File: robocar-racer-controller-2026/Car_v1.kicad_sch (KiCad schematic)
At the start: 36 parts, among them J1 GY-87, J10 Buck in, J11 Motor_in, J12 Bateria 3s, J13 Buck_out, J14 Raspbery_usbc, J15 Step_up, J16 Radio, J3 Sinal_Servo, J4 Sinal_Motor, J5 Conn_01x19_Socket, J6 Conn_01x19_Socket, J7 Serial, J8 ADS1115, J9 Bateria 2s, SW1 SW_DPST_x2, SW2 SW_DPST_x2, U2 ESP32-DEVKITC-32D

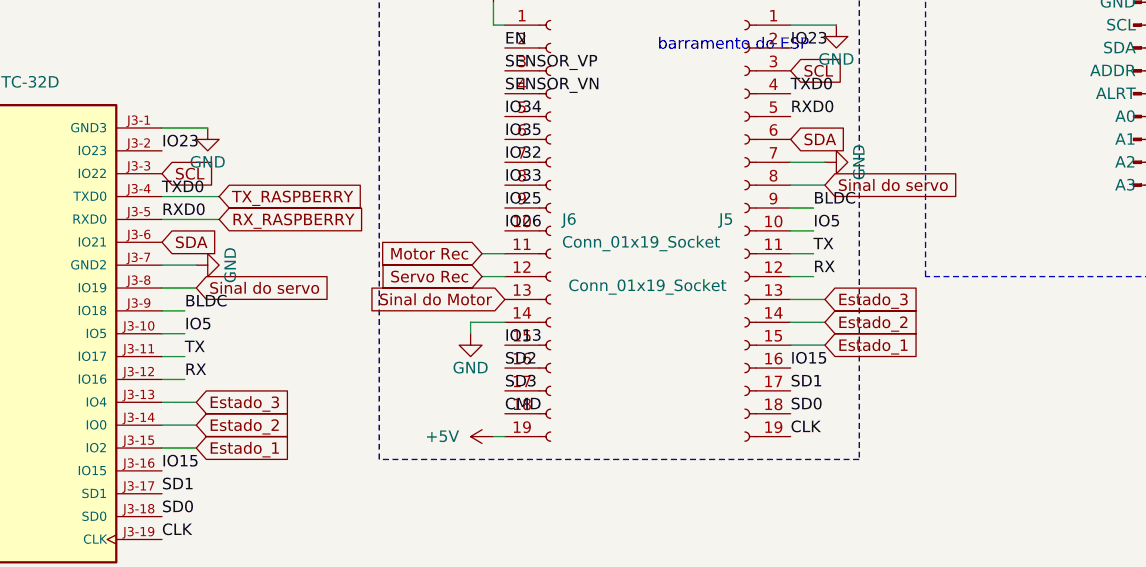
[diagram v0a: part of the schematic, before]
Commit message: ajustes na entrada serial
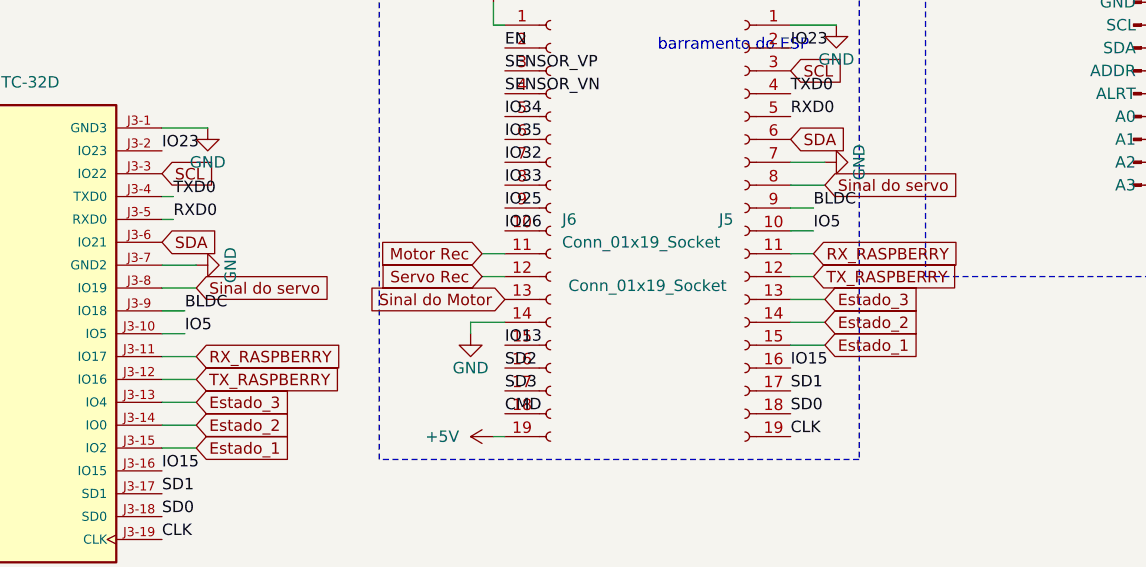
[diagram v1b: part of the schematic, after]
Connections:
- net RX is gone; now on net TX_RASPBERRY: J5.12 (Pin_12), U2.J3-12 (IO16)
- net TX is gone; now on net RX_RASPBERRY: J5.11 (Pin_11), U2.J3-11 (IO17)
- net RX_RASPBERRY: no longer J5.5 (Pin_5), U2.J3-5 (RXD0)
- net TX_RASPBERRY: no longer J5.4 (Pin_4), U2.J3-4 (TXD0)
- new net RXD0: J5.5 (Pin_5), U2.J3-5 (RXD0)
- new net TXD0: J5.4 (Pin_4), U2.J3-4 (TXD0)
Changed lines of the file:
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@@
-	(wire
-		(pts
-			(xy 132.08 135.89) (xy 138.43 135.89)
-		)
-		(stroke
-			(width 0)
-			(type default)
-		)
-	)
 	(wire
 		(pts
@@
 	(wire
 		(pts
+			(xy 132.08 156.21) (xy 135.89 156.21)
+		)
+		(stroke
+			(width 0)
+			(type default)
+		)
+	)
+	(wire
+		(pts
+			(xy 132.08 153.67) (xy 135.89 153.67)
+		)
+		(stroke
+			(width 0)
+			(type default)
+		)
+	)
+	(wire
+		(pts
 			(xy 168.91 116.84) (xy 170.18 116.84)
 		)
@@
 	(wire
 		(pts
+			(xy 133.35 138.43) (xy 132.08 138.43)
+		)
+		(stroke
+			(width 0)
+			(type default)
+		)
+	)
+	(wire
+		(pts
 			(xy 62.23 124.46) (xy 62.23 119.38)
 		)
@@
 	(wire
 		(pts
-			(xy 132.08 138.43) (xy 138.43 138.43)
-		)
-		(stroke
-			(width 0)
-			(type default)
-		)
-	)
-	(wire
-		(pts
 			(xy 168.91 162.56) (xy 170.18 162.56)
 		)
@@
 	(wire
 		(pts
-			(xy 134.62 153.67) (xy 132.08 153.67)
-		)
-		(stroke
-			(width 0)
-			(type default)
-		)
-	)
-	(wire
-		(pts
 			(xy 245.11 127) (xy 246.38 127)
 		)
@@
 	(wire
 		(pts
+			(xy 133.35 135.89) (xy 132.08 135.89)
+		)
+		(stroke
+			(width 0)
+			(type default)
+		)
+	)
+	(wire
+		(pts
 			(xy 36.83 180.34) (xy 34.29 180.34)
 		)
@@
 		(pts
 			(xy 204.47 137.16) (xy 201.93 137.16)
-		)
-		(stroke
-			(width 0)
-			(type default)
-		)
-	)
-	(wire
-		(pts
-			(xy 132.08 156.21) (xy 134.62 156.21)
 		)
 		(stroke
@@
 		)
 	)
-	(label "RXD0"
-		(at 132.08 138.43 0)
-		(effects
-			(font
-				(size 1.27 1.27)
-			)
-			(justify left bottom)
-		)
-	)
 	(label "EN"
 		(at 170.18 119.38 0)
@@
 	)
 	(label "TXD0"
-		(at 132.08 135.89 0)
-		(effects
-			(font
-				(size 1.27 1.27)
-			)
-			(justify left bottom)
-		)
-	)
-	(label "TX"
-		(at 204.47 142.24 0)
+		(at 133.35 135.89 0)
 		(effects
 			(font
@@
 		)
 	)
-	(label "RX"
-		(at 134.62 156.21 0)
-		(effects
-			(font
-				(size 1.27 1.27)
-			)
-			(justify left bottom)
-		)
-	)
 	(label "IO26"
 		(at 91.44 151.13 0)
@@
 		)
 	)
-	(label "TX"
-		(at 134.62 153.67 0)
-		(effects
-			(font
-				(size 1.27 1.27)
-			)
-			(justify left bottom)
-		)
-	)
 	(label "CLK"
 		(at 201.93 162.56 0)
@@
 		)
 	)
+	(label "RXD0"
+		(at 133.35 138.43 0)
+		(effects
+			(font
+				(size 1.27 1.27)
+			)
+			(justify left bottom)
+		)
+	)
 	(label "IO32"
 		(at 170.18 132.08 0)
@@
 	(label "SD0"
 		(at 201.93 160.02 0)
-		(effects
-			(font
-				(size 1.27 1.27)
-			)
-			(justify left bottom)
-		)
-	)
-	(label "RX"
-		(at 204.47 144.78 0)
 		(effects
 			(font
@@
 	(global_label "TX_RASPBERRY"
 		(shape input)
+		(at 204.47 144.78 0)
+		(fields_autoplaced yes)
+		(effects
+			(font
+				(size 1.27 1.27)
+			)
+			(justify left)
+		)
+		(property "Intersheetrefs" "${INTERSHEET_REFS}"
+			(at 221.4856 144.78 0)
+			(hide yes)
+			(show_name no)
+			(do_not_autoplace no)
+			(effects
+				(font
+					(size 1.27 1.27)
+				)
+				(justify left)
+			)
+		)
+	)
+	(global_label "TX_RASPBERRY"
+		(shape input)
 		(at 241.3 60.96 0)
 		(fields_autoplaced yes)
@@
 	(global_label "RX_RASPBERRY"
 		(shape input)
-		(at 138.43 138.43 0)
+		(at 135.89 153.67 0)
 		(fields_autoplaced yes)
 		(effects
@@
 		)
 		(property "Intersheetrefs" "${INTERSHEET_REFS}"
-			(at 155.748 138.43 0)
+			(at 153.208 153.67 0)
 			(hide yes)
 			(show_name no)
@@
 		)
 	)
+	(global_label "RX_RASPBERRY"
+		(shape input)
+		(at 204.47 142.24 0)
+		(fields_autoplaced yes)
+		(effects
+			(font
+				(size 1.27 1.27)
+			)
+			(justify left)
+		)
+		(property "Intersheetrefs" "${INTERSHEET_REFS}"
+			(at 221.788 142.24 0)
+			(hide yes)
+			(show_name no)
+			(do_not_autoplace no)
+			(effects
+				(font
+					(size 1.27 1.27)
+				)
+				(justify left)
+			)
+		)
+	)
 	(global_label "TX_RASPBERRY"
 		(shape input)
-		(at 138.43 135.89 0)
+		(at 135.89 156.21 0)
 		(fields_autoplaced yes)
 		(effects
@@
 		)
 		(property "Intersheetrefs" "${INTERSHEET_REFS}"
-			(at 155.4456 135.89 0)
+			(at 152.9056 156.21 0)
 			(hide yes)
 			(show_name no)
